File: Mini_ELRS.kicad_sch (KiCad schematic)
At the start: 24 parts, among them J1 Conn_01x06, J2 Conn_01x06, J3 Conn_01x06, SW1 SW_Push, U1 ESP32-PICO-D4, U2 TC2014-3.3VxCTTR, U3 SX1280IMLTRT, Y1 Crystal_GND24_Small

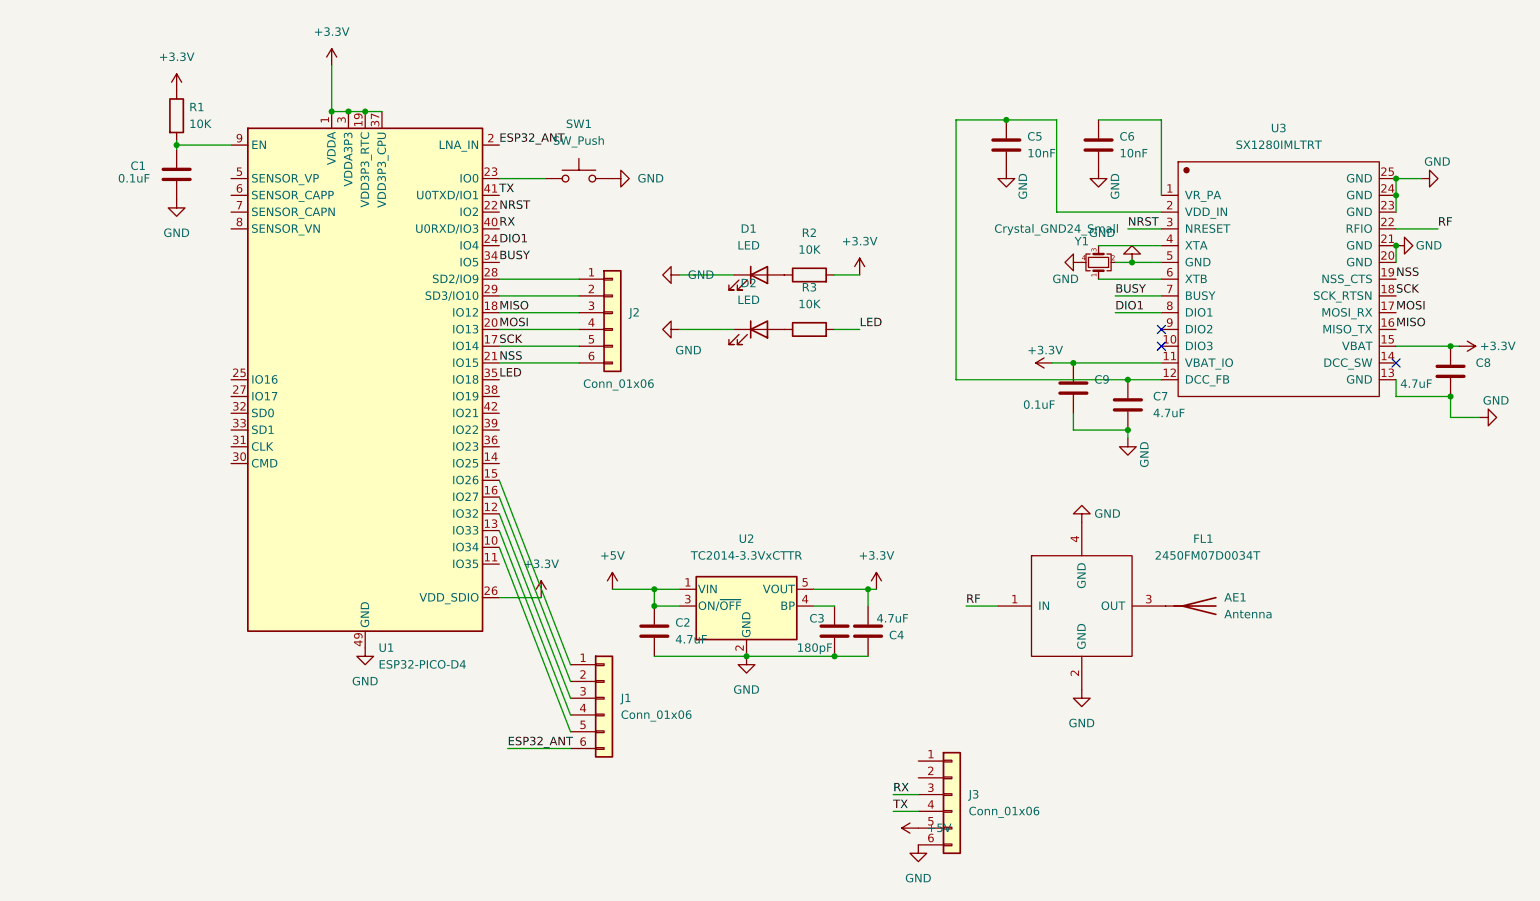
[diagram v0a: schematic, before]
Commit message: stash for esp8266
Signed-off-by: ncerzzk <huangzzk@bupt.edu.cn>
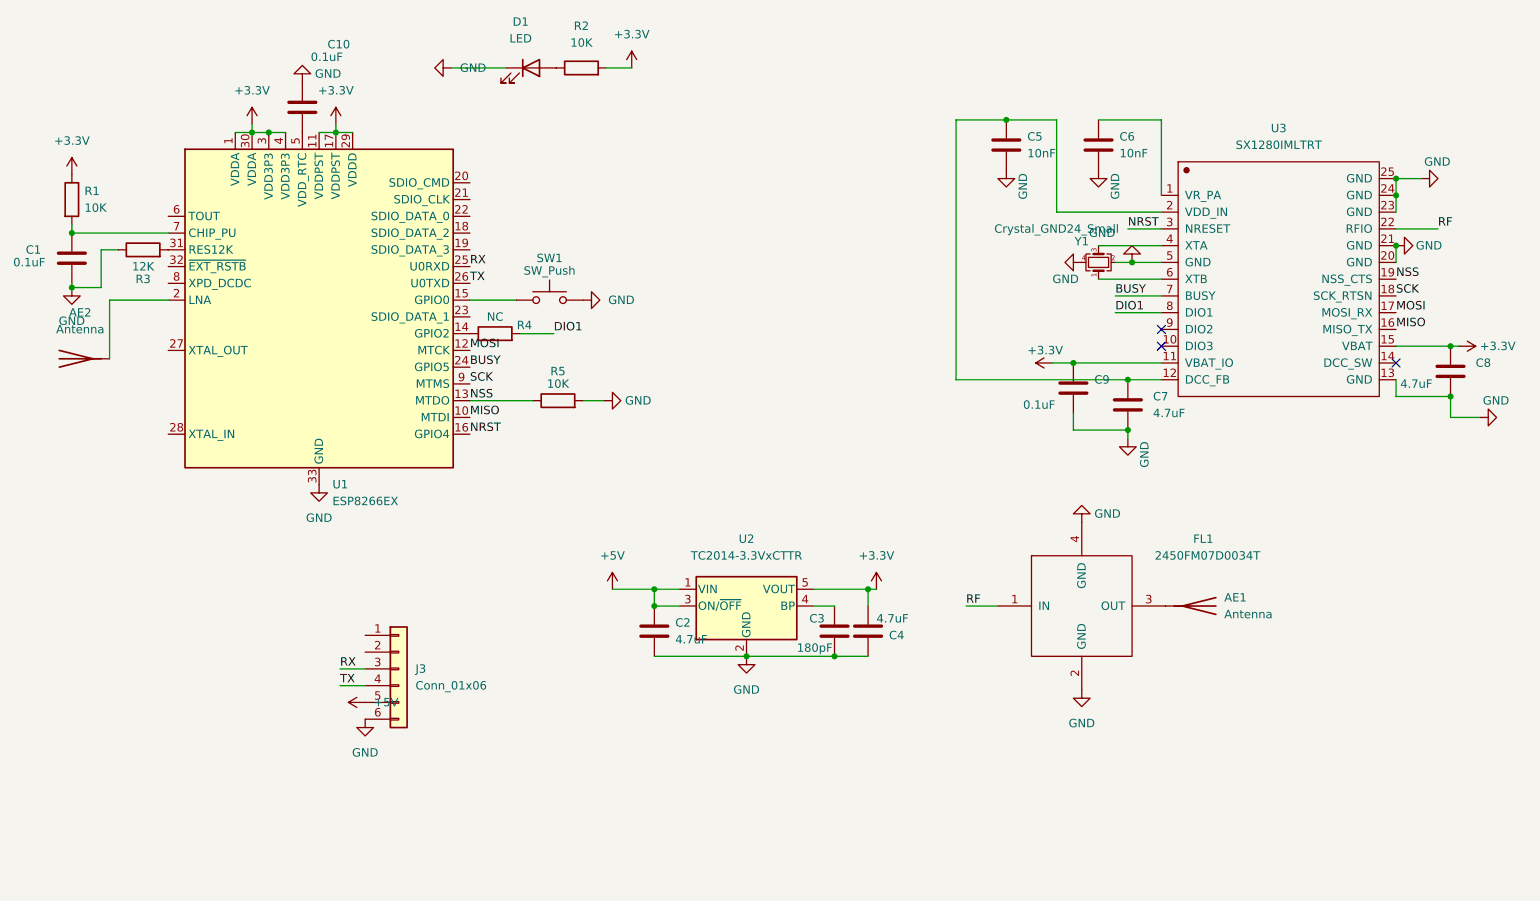
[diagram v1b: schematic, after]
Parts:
- removed D2: LED, LED_SMD:LED_0603_1608Metric, symbol Device:LED
- removed J1, J2: Conn_01x06, Connector_PinHeader_2.54mm:PinHeader_1x06_P2.54mm_Vertical, symbol Connector_Generic:Conn_01x06
- removed U1: ESP32-PICO-D4, Package_DFN_QFN:QFN-48-1EP_7x7mm_P0.5mm_EP5.3x5.3mm, symbol RF_Module:ESP32-PICO-D4
- added AE2: Antenna, RF_Antenna:Texas_SWRA117D_2.4GHz_Left, symbol Device:Antenna
- added C10: 0.1uF, Capacitor_SMD:C_0402_1005Metric, symbol Device:C
- added R4: NC, Resistor_SMD:R_0402_1005Metric, symbol Device:R
- added R5: 10K, Resistor_SMD:R_0402_1005Metric, symbol Device:R
- added U1: ESP8266EX, Package_DFN_QFN:QFN-32-1EP_5x5mm_P0.5mm_EP3.45x3.45mm, symbol MCU_Espressif:ESP8266EX
- C1, C2, C3, C4, C5, C6, C7, C8, C9: footprint Capacitor_SMD:C_0603_1608Metric -> Capacitor_SMD:C_0402_1005Metric
- R1, R2: footprint Resistor_SMD:R_0603_1608Metric -> Resistor_SMD:R_0402_1005Metric
- R3: value 10K -> 12K; footprint Resistor_SMD:R_0603_1608Metric -> Resistor_SMD:R_0402_1005Metric
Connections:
- net +3V3: now also U1.1 (VDDA), U1.11 (VDDPST), U1.17 (VDDPST), U1.29 (VDDD), U1.3 (VDD3P3), U1.30 (VDDA), U1.4 (VDD3P3)
- net BUSY: now also U1.24 (GPIO5)
- net DIO1: now also R4.2
- net GND: now also R3.1, C10.1, R5.2, U1.33 (GND)
- net MISO: now also U1.10 (MTDI)
- net MOSI: now also U1.12 (MTCK)
- net NRST: now also U1.16 (GPIO4)
- net NSS: now also R5.1, U1.13 (MTDO)
- net RX: now also U1.25 (U0RXD)
- net SCK: now also U1.9 (MTMS)
- net TX: now also U1.26 (U0TXD)
- net at C1.1, R1.2: now also U1.7 (CHIP_PU)
- net at SW1.1: now also U1.15 (GPIO0)
- net LED: no longer names the net of R3.2
- net LED: now also U1.31 (RES12K)
- new net: AE2.1 (A), U1.2 (LNA)
- new net: R4.1, U1.14 (GPIO2)
- new net: C10.2, U1.5 (VDD_RTC)
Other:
- moved on the sheet: C1, D1, J3, R1, R2, SW1
